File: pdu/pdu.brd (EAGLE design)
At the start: 17.5 x 90 mm, 62 parts, among them IC1 FDN359BN, IC2 FDN359BN, IC3 FDN359BN, J1 S2B-PH-K-S(LF)(SN), J10 S2B-PH-K-S(LF)(SN), J2 S2B-PH-K-S(LF)(SN), J3 S2B-PH-K-S(LF)(SN), J4 S2B-PH-K-S(LF)(SN), J5 S2B-PH-K-S(LF)(SN), J6 S2B-PH-K-S(LF)(SN), J7 S2B-PH-K-S(LF)(SN), J8 S2B-PH-K-S(LF)(SN), J9 S2B-PH-K-S(LF)(SN)

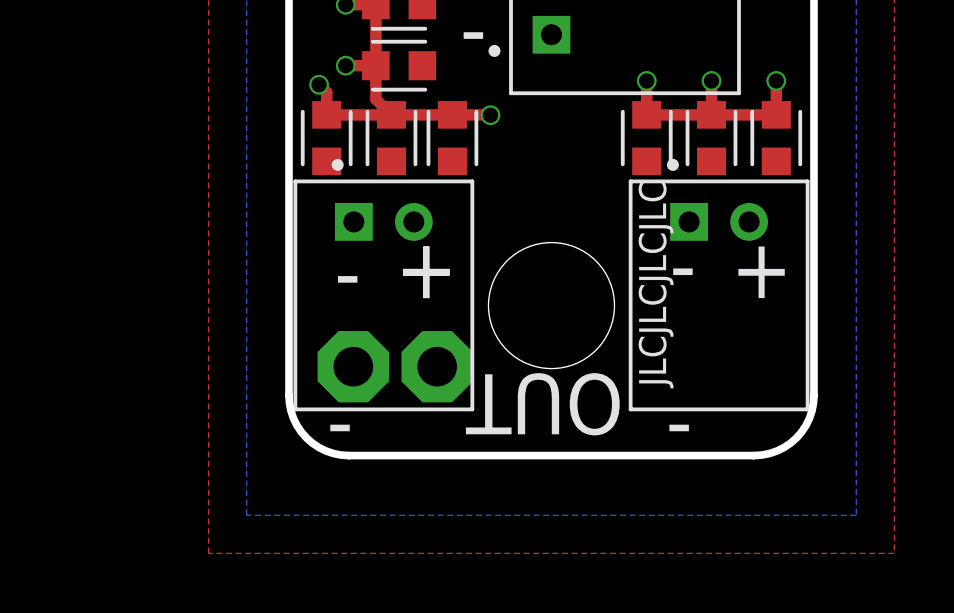
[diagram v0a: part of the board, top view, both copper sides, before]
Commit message: graphics improvements
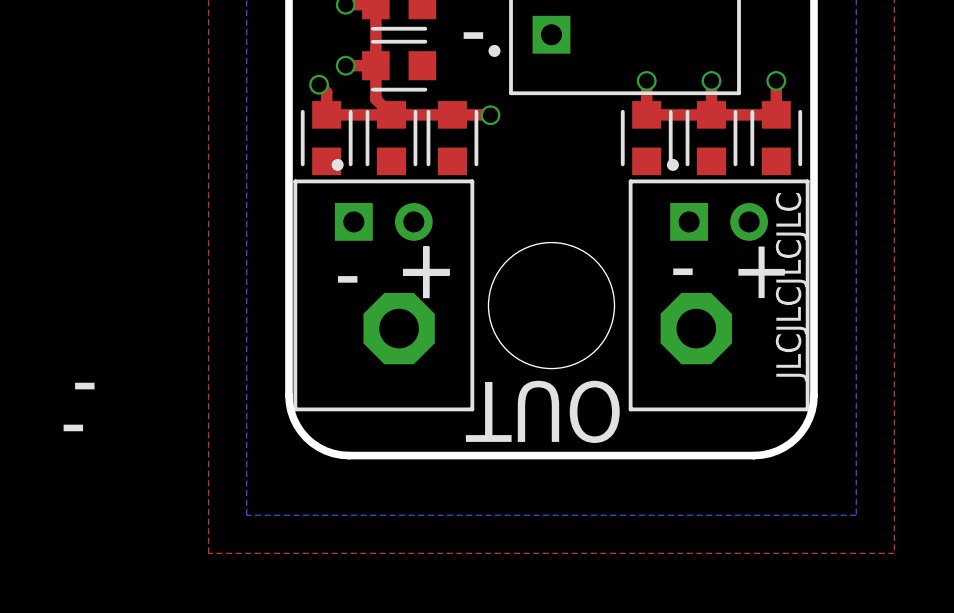
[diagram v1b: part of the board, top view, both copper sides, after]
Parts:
- moved TP1 11.5 mm to (4.83, -40.8)
- moved TP2 1.80 mm to (-5.08, -40.8)
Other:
- board text added: "Designed by ART Avionics"
- board text added: "Shrey Bohra Shreya Ramteke Sharwa Molla Abhik Chatterjee Camillo De Gregorio"

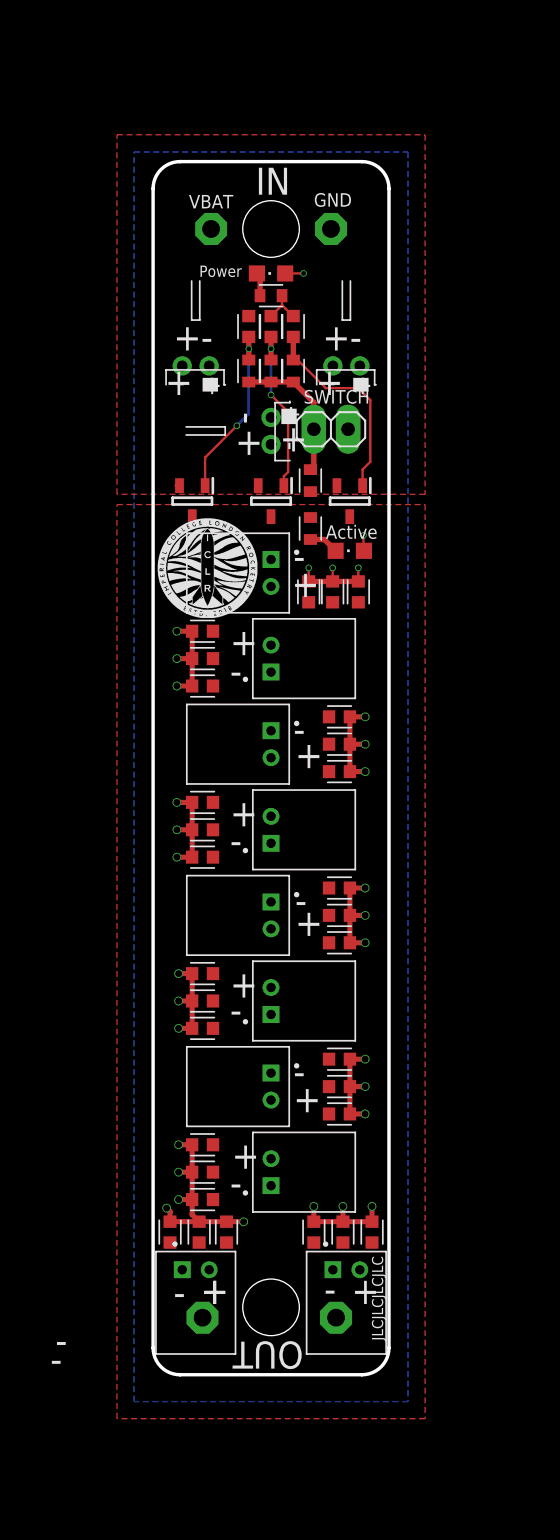
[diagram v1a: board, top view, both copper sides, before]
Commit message: export new pdu
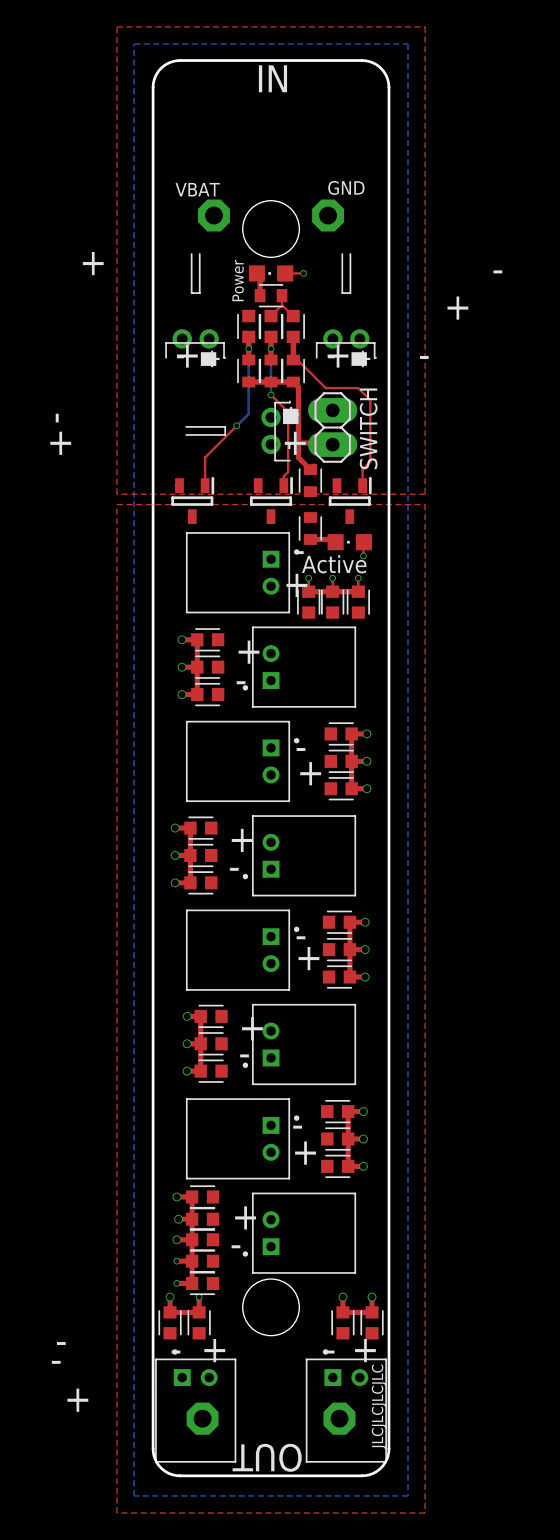
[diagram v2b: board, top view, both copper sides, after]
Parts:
- moved C7 9.09 mm to (-5.08, -38.2), turned to 180 degrees
- moved J1 8.00 mm to (5.59, -45.2)
- moved J2 8.00 mm to (-5.59, -45.2)
- moved TP1 7.50 mm to (5.08, -48.3)
- moved TP2 7.49 mm to (-5.08, -48.3)
- moved C4 6.73 mm to (-7.49, -41.1)
- moved C5 6.73 mm to (-5.33, -41.1)
- moved C8 6.73 mm to (5.33, -41.1)
- moved C9 6.73 mm to (7.49, -41.1)
- moved J10 4.53 mm to (0.00, -34.5)
- moved C23 3.89 mm to (4.95, -29.5)
- moved C24 3.89 mm to (4.95, -27.5)
- moved C25 3.89 mm to (4.95, -25.5)
- moved J9 3.88 mm to (0.00, -27.5)
- moved C10 3.87 mm to (-5.08, -31.8)
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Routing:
- net EN: track 10.5 -> 13.3 mm
- net VBAT: track 77.0 -> 74.4 mm, vias 31 -> 32
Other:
- board size 17.5 x 90 mm -> 17.5 x 105 mm
- board text added: ".05"
- board text added: "100"
- board text added: "3.5"
- board text added: "90"
- board text added: "95"
- board text added: "Shrey Bohra Shreya Ramteke Sharwa Molla Hritik Parmessur Abhik Chatterjee Camillo De Gregorio Ella Devesa"
- board text removed: "0.05"
- board text removed: "Shrey Bohra Shreya Ramteke Sharwa Molla Abhik Chatterjee Camillo De Gregorio"
